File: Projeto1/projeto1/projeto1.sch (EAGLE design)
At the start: 2 parts

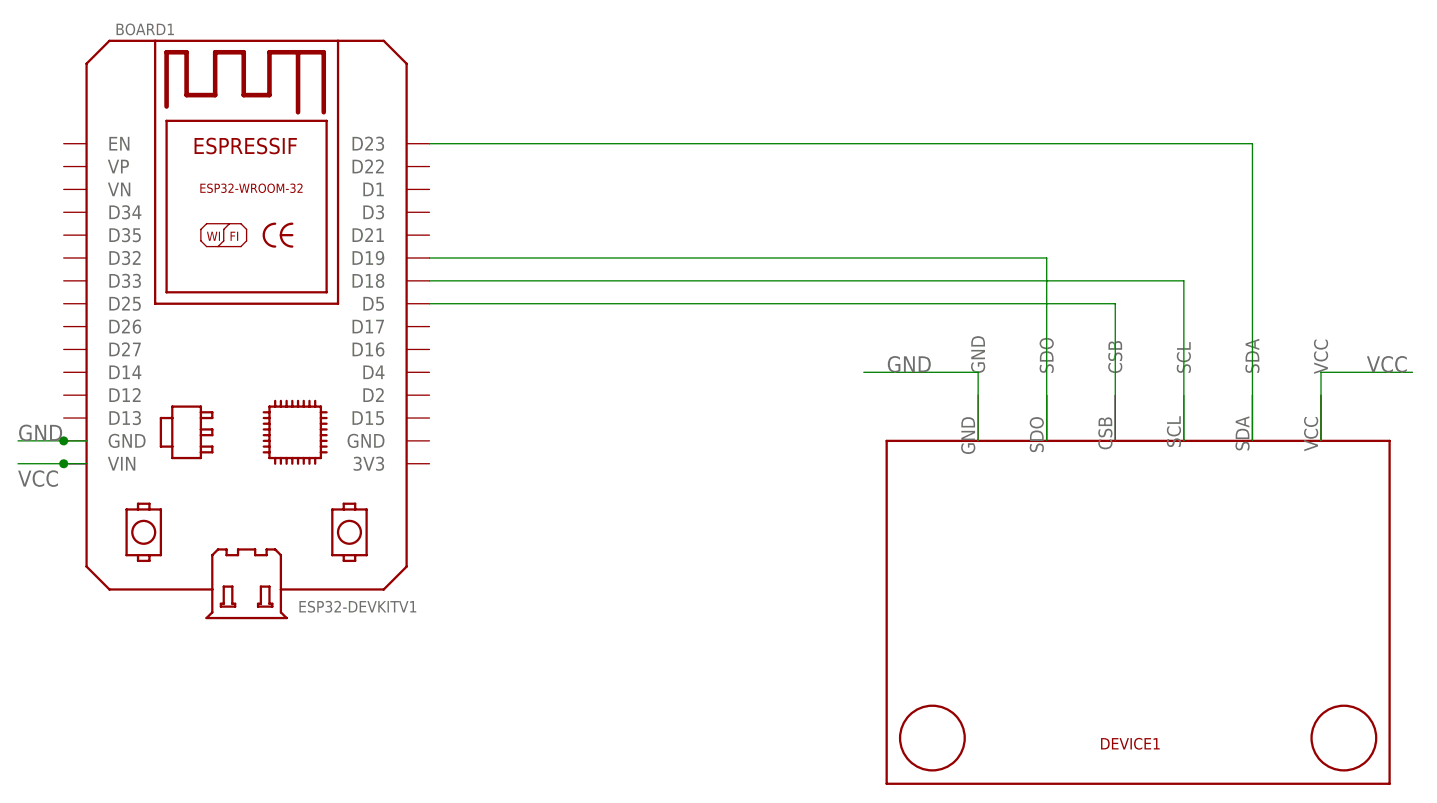
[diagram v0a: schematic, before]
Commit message: Add files via upload
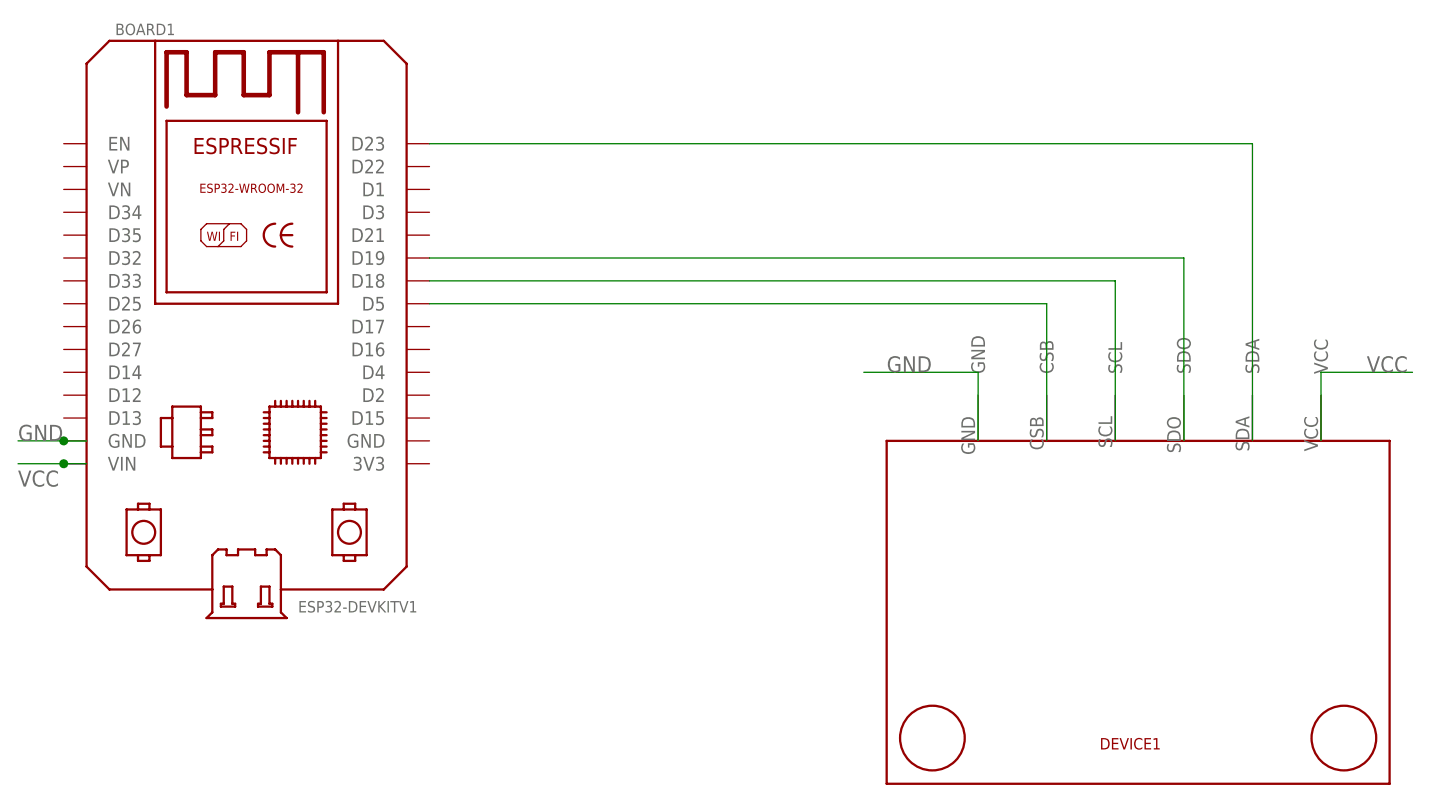
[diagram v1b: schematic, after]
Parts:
- renumbered U$1 to U$2
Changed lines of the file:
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@@
 <setting verticaltext="up"/>
 </settings>
-<grid distance="0.1" unitdist="inch" unit="mm" style="lines" multiple="1" display="yes" altdistance="0.01" altunitdist="inch" altunit="mm"/>
+<grid distance="0.1" unitdist="inch" unit="inch" style="lines" multiple="1" display="no" altdistance="0.01" altunitdist="inch" altunit="inch"/>
 <layers>
 <layer number="1" name="Top" color="4" fill="1" visible="no" active="no"/>
@@
 <parts>
 <part name="FRAME1" library="frames" library_urn="urn:adsk.eagle:library:229" deviceset="A4L-LOC" device=""/>
-<part name="U$1" library="Cactus_Library" deviceset="DEVICE1" device=""/>
 <part name="BOARD1" library="ESP32-DEVKITV1" deviceset="ESP32DEVKITV1" device=""/>
+<part name="U$2" library="Cactus_Library" deviceset="DEVICE1" device=""/>
 </parts>
 <sheets>
@@
 <attribute name="SHEET" x="225.425" y="-2.54" size="2.54" layer="94"/>
 </instance>
-<instance part="U$1" gate="G$1" x="185.42" y="38.1" smashed="yes" rot="R180"/>
 <instance part="BOARD1" gate="G$1" x="68.58" y="45.72" smashed="yes">
 <attribute name="NAME" x="71.755" y="103.505" size="1.27" layer="95"/>
 </instance>
+<instance part="U$2" gate="G$1" x="185.42" y="38.1" smashed="yes" rot="R180"/>
 </instances>
 <busses>
@@
 </segment>
 <segment>
-<pinref part="U$1" gate="G$1" pin="GND"/>
 <wire x1="167.64" y1="58.42" x2="167.64" y2="66.04" width="0.1524" layer="91"/>
 <label x="157.48" y="66.04" size="1.778" layer="95"/>
 <wire x1="167.64" y1="66.04" x2="154.94" y2="66.04" width="0.1524" layer="91"/>
+<pinref part="U$2" gate="G$1" pin="GND"/>
 </segment>
 </net>
 <net name="N$1" class="0">
 <segment>
-<pinref part="U$1" gate="G$1" pin="SDA"/>
 <wire x1="198.12" y1="58.42" x2="198.12" y2="91.44" width="0.1524" layer="91"/>
 <pinref part="BOARD1" gate="G$1" pin="D23"/>
 <wire x1="198.12" y1="91.44" x2="106.68" y2="91.44" width="0.1524" layer="91"/>
+<pinref part="U$2" gate="G$1" pin="SDA"/>
 </segment>
 </net>
 <net name="N$5" class="0">
 <segment>
-<pinref part="U$1" gate="G$1" pin="CSB"/>
-<wire x1="182.88" y1="58.42" x2="182.88" y2="73.66" width="0.1524" layer="91"/>
+<wire x1="182.88" y1="58.42" x2="182.88" y2="76.2" width="0.1524" layer="91"/>
+<pinref part="U$2" gate="G$1" pin="SCL"/>
+<pinref part="BOARD1" gate="G$1" pin="D18"/>
+<wire x1="182.88" y1="76.2" x2="106.68" y2="76.2" width="0.1524" layer="91"/>
+</segment>
+</net>
+<net name="N$2" class="0">
+<segment>
+<pinref part="U$2" gate="G$1" pin="CSB"/>
 <pinref part="BOARD1" gate="G$1" pin="D5"/>
-<wire x1="106.68" y1="73.66" x2="182.88" y2="73.66" width="0.1524" layer="91"/>
-</segment>
-</net>
-<net name="N$2" class="0">
-<segment>
-<pinref part="U$1" gate="G$1" pin="SDO"/>
-<wire x1="175.26" y1="78.74" x2="175.26" y2="58.42" width="0.1524" layer="91"/>
+<wire x1="175.26" y1="73.66" x2="175.26" y2="58.42" width="0.1524" layer="91"/>
+<wire x1="106.68" y1="73.66" x2="175.26" y2="73.66" width="0.1524" layer="91"/>
+</segment>
+</net>
+<net name="N$3" class="0">
+<segment>
+<wire x1="190.5" y1="78.74" x2="190.5" y2="58.42" width="0.1524" layer="91"/>
+<pinref part="U$2" gate="G$1" pin="SDO"/>
 <pinref part="BOARD1" gate="G$1" pin="D19"/>
-<wire x1="175.26" y1="78.74" x2="106.68" y2="78.74" width="0.1524" layer="91"/>
-</segment>
-</net>
-<net name="N$3" class="0">
-<segment>
-<pinref part="U$1" gate="G$1" pin="SCL"/>
-<pinref part="BOARD1" gate="G$1" pin="D18"/>
-<wire x1="190.5" y1="76.2" x2="190.5" y2="58.42" width="0.1524" layer="91"/>
-<wire x1="190.5" y1="76.2" x2="106.68" y2="76.2" width="0.1524" layer="91"/>
+<wire x1="106.68" y1="78.74" x2="190.5" y2="78.74" width="0.1524" layer="91"/>
 </segment>
 </net>
@@
 </segment>
 <segment>
-<pinref part="U$1" gate="G$1" pin="VCC"/>
 <wire x1="205.74" y1="58.42" x2="205.74" y2="66.04" width="0.1524" layer="91"/>
 <wire x1="205.74" y1="66.04" x2="215.9" y2="66.04" width="0.1524" layer="91"/>
 <label x="210.82" y="66.04" size="1.778" layer="95"/>
-</segment>
-</net>
+<pinref part="U$2" gate="G$1" pin="VCC"/>
+</segment>
+</net>
